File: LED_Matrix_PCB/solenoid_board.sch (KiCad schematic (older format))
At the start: 93 parts, among them J2 MCU_LEFT_LEGS, J3 MCU_RIGHT_LEGS

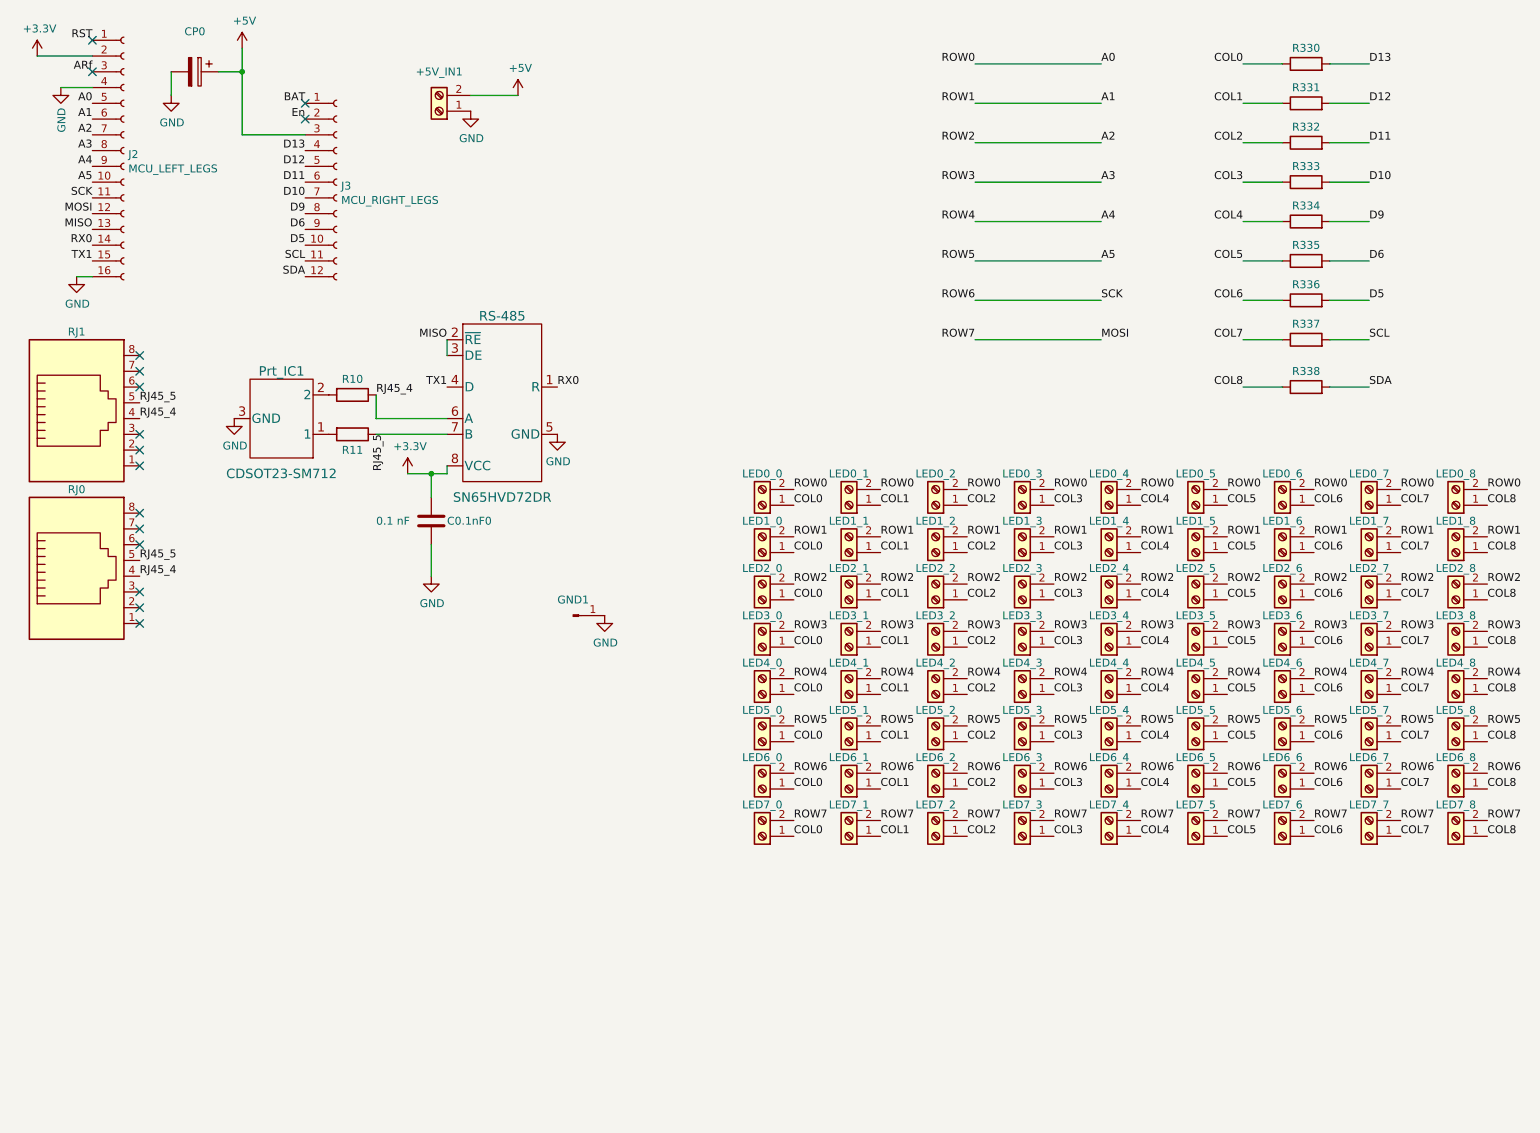
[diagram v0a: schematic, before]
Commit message: Forgot to close files before pushing.
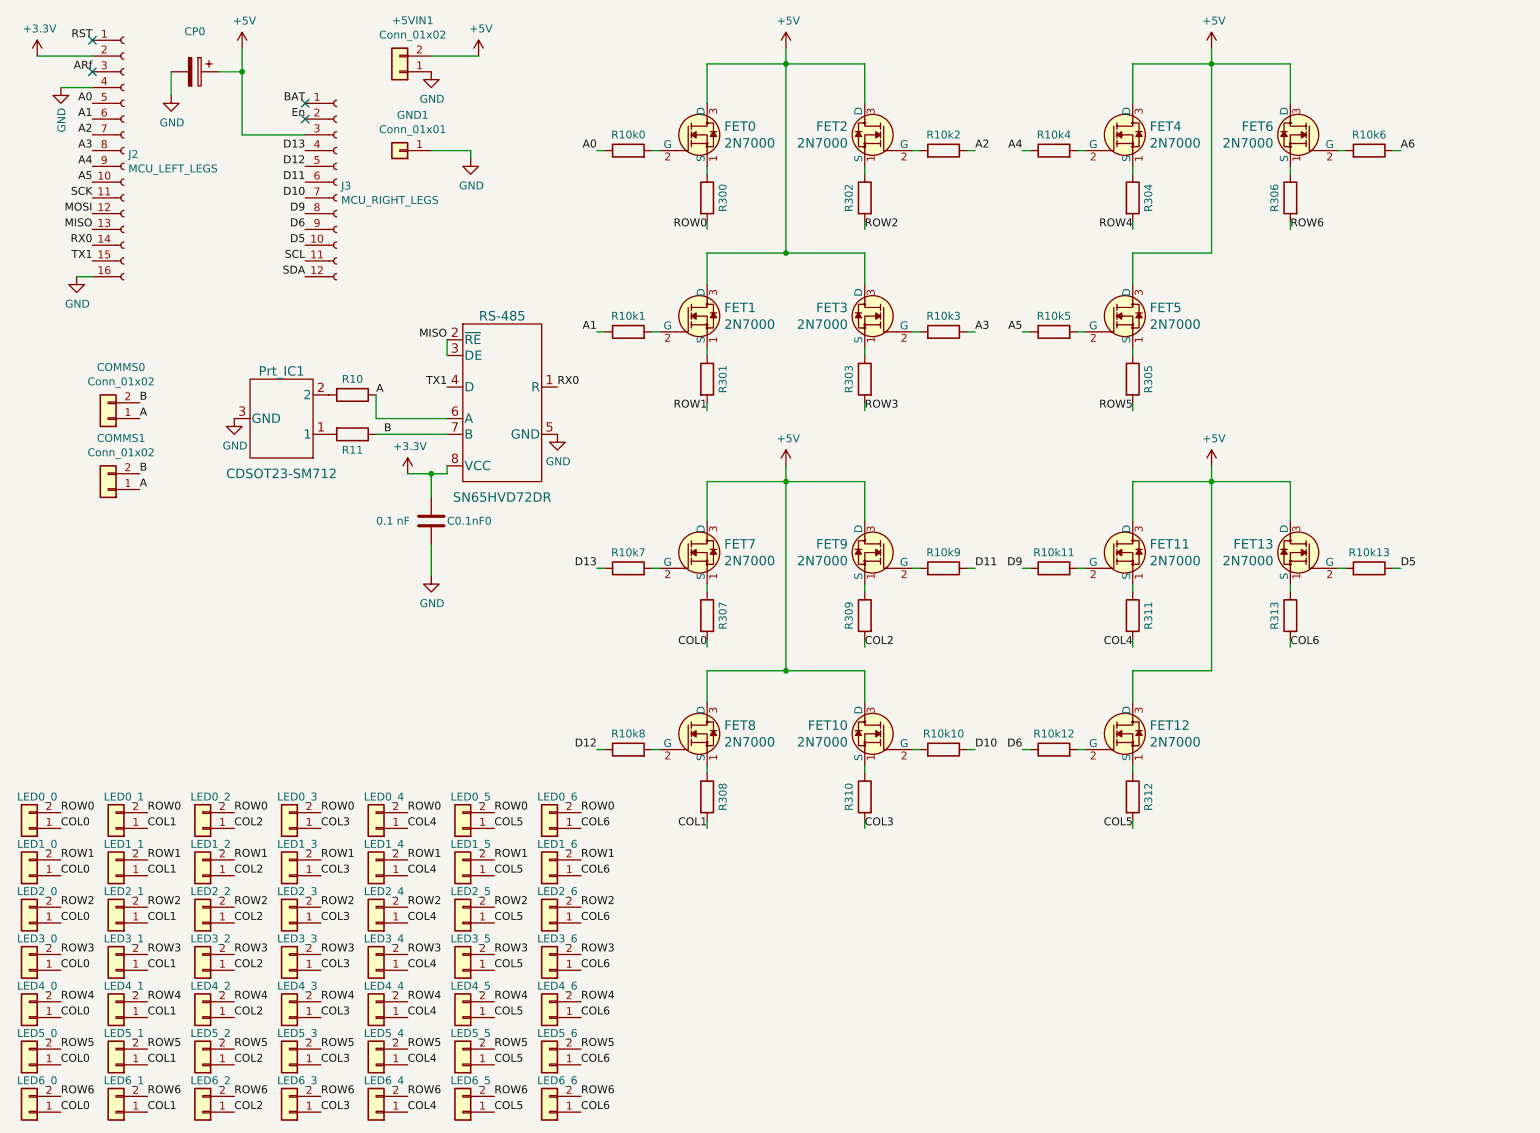
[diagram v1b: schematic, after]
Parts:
- removed +5V_IN1: MCU_PWR_Supply, TerminalBlock:TerminalBlock_bornier-2_P5.08mm, symbol Connector:Screw_Terminal_01x02
- removed GND1: Conn_01x01_Male, Connector_PinHeader_2.54mm:PinHeader_1x01_P2.54mm_Vertical, symbol Connector:Conn_01x01_Male
- removed LED0_0, LED0_1, LED0_2, LED0_3, LED0_4, LED0_5, LED0_6, LED0_7, LED0_8, LED1_0, LED1_1, LED1_2, LED1_3, LED1_4, LED1_5, LED1_6, LED1_7, LED1_8, LED2_0, LED2_1, LED2_2, LED2_3, LED2_4, LED2_5, LED2_6, LED2_7, LED2_8, LED3_0, LED3_1, LED3_2, LED3_3, LED3_4, LED3_5, LED3_6, LED3_7, LED3_8, LED4_0, LED4_1, LED4_2, LED4_3, LED4_4, LED4_5, LED4_6, LED4_7, LED4_8, LED5_0, LED5_1, LED5_2, LED5_3, LED5_4, LED5_5, LED5_6, LED5_7, LED5_8, LED6_0, LED6_1, LED6_2, LED6_3, LED6_4, LED6_5, LED6_6, LED6_7, LED6_8, LED7_0, LED7_1, LED7_2, LED7_3, LED7_4, LED7_5, LED7_6, LED7_7, LED7_8: Screw-terminal, TerminalBlock:TerminalBlock_bornier-2_P5.08mm, symbol Connector:Screw_Terminal_01x02
- removed R330, R331, R332: 330, Resistor_THT:R_Axial_DIN0309_L9.0mm_D3.2mm_P20.32mm_Horizontal, symbol Device:R
- removed R333, R334, R335, R336, R337, R338: R, Resistor_THT:R_Axial_DIN0309_L9.0mm_D3.2mm_P20.32mm_Horizontal, symbol Device:R
- removed RJ0, RJ1: RJ45, Connector_RJ:RJ45_Amphenol_54602-x08_Horizontal, symbol Connector:RJ45
- added +5VIN1, COMMS0, COMMS1, LED0_0, LED0_1, LED0_2, LED0_3, LED0_4, LED0_5, LED0_6, LED1_0, LED1_1, LED1_2, LED1_3, LED1_4, LED1_5, LED1_6, LED2_0, LED2_1, LED2_2, LED2_3, LED2_4, LED2_5, LED2_6, LED3_0, LED3_1, LED3_2, LED3_3, LED3_4, LED3_5, LED3_6, LED4_0, LED4_1, LED4_2, LED4_3, LED4_4, LED4_5, LED4_6, LED5_0, LED5_1, LED5_2, LED5_3, LED5_4, LED5_5, LED5_6, LED6_0, LED6_1, LED6_2, LED6_3, LED6_4, LED6_5, LED6_6: Conn_01x02, Connector_PinHeader_2.54mm:PinHeader_1x02_P2.54mm_Vertical, symbol Connector_Generic:Conn_01x02
- added FET0, FET1, FET10, FET11, FET12, FET13, FET2, FET3, FET4, FET5, FET6, FET7, FET8, FET9: 2N7000, digikey-footprints:TO-92-3, symbol dk_Transistors-FETs-MOSFETs-Single:2N7000
- added GND1: Conn_01x01, Connector_PinHeader_2.54mm:PinHeader_1x01_P2.54mm_Vertical, symbol Connector_Generic:Conn_01x01
- added R10k0, R10k1, R10k10, R10k11, R10k12, R10k13, R10k2, R10k3, R10k4, R10k5, R10k6, R10k7, R10k8, R10k9: 10k, Resistor_THT:R_Axial_DIN0204_L3.6mm_D1.6mm_P5.08mm_Vertical, symbol Device:R
- added R300, R301, R302, R303, R304, R305, R306, R307, R308, R309, R310, R311, R312, R313: 300, Resistor_THT:R_Axial_DIN0204_L3.6mm_D1.6mm_P5.08mm_Vertical, symbol Device:R
- R10, R11: footprint Resistor_THT:R_Axial_DIN0309_L9.0mm_D3.2mm_P20.32mm_Horizontal -> Resistor_THT:R_Axial_DIN0204_L3.6mm_D1.6mm_P7.62mm_Horizontal
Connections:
- net +5V: now also +5VIN1.2 (Pin_2), FET0.3 (D), FET1.3 (D), FET10.3 (D), FET11.3 (D), FET12.3 (D), FET13.3 (D), FET2.3 (D), FET3.3 (D), FET4.3 (D), FET5.3 (D), FET6.3 (D), FET7.3 (D), FET8.3 (D), FET9.3 (D)
- net A0: now also R10k0.1
- net A1: now also R10k1.1
- net A2: now also R10k2.1
- net A3: now also R10k3.1
- net A4: now also R10k4.1
- net A5: now also R10k5.1
- net COL0: now also LED0_0.1 (Pin_1), LED1_0.1 (Pin_1), LED2_0.1 (Pin_1), LED3_0.1 (Pin_1), LED4_0.1 (Pin_1), LED5_0.1 (Pin_1), LED6_0.1 (Pin_1), R307.2
- net COL1: now also LED0_1.1 (Pin_1), LED1_1.1 (Pin_1), LED2_1.1 (Pin_1), LED3_1.1 (Pin_1), LED4_1.1 (Pin_1), LED5_1.1 (Pin_1), LED6_1.1 (Pin_1), R308.2
- net COL2: now also LED0_2.1 (Pin_1), LED1_2.1 (Pin_1), LED2_2.1 (Pin_1), LED3_2.1 (Pin_1), LED4_2.1 (Pin_1), LED5_2.1 (Pin_1), LED6_2.1 (Pin_1), R309.2
- net COL3: now also LED0_3.1 (Pin_1), LED1_3.1 (Pin_1), LED2_3.1 (Pin_1), LED3_3.1 (Pin_1), LED4_3.1 (Pin_1), LED5_3.1 (Pin_1), LED6_3.1 (Pin_1), R310.2
- net COL4: now also LED0_4.1 (Pin_1), LED1_4.1 (Pin_1), LED2_4.1 (Pin_1), LED3_4.1 (Pin_1), LED4_4.1 (Pin_1), LED5_4.1 (Pin_1), LED6_4.1 (Pin_1), R311.2
- net COL5: now also LED0_5.1 (Pin_1), LED1_5.1 (Pin_1), LED2_5.1 (Pin_1), LED3_5.1 (Pin_1), LED4_5.1 (Pin_1), LED5_5.1 (Pin_1), LED6_5.1 (Pin_1), R312.2
- net COL6: now also LED0_6.1 (Pin_1), LED1_6.1 (Pin_1), LED2_6.1 (Pin_1), LED3_6.1 (Pin_1), LED4_6.1 (Pin_1), LED5_6.1 (Pin_1), LED6_6.1 (Pin_1), R313.2
- net D10: now also R10k10.1
- net D11: now also R10k9.1
- net D12: now also R10k8.1
- net D13: now also R10k7.1
- net D5: now also R10k13.1
- net D6: now also R10k12.1
- net D9: now also R10k11.1
- net GND: now also +5VIN1.1 (Pin_1), GND1.1 (Pin_1)
- net ROW6: now also LED6_0.2 (Pin_2), LED6_1.2 (Pin_2), LED6_2.2 (Pin_2), LED6_3.2 (Pin_2), LED6_4.2 (Pin_2), LED6_5.2 (Pin_2), LED6_6.2 (Pin_2), R306.2; no longer J2.11 (Pin_11)
- net RJ45_4 renamed A
- net A: now also COMMS0.1 (Pin_1), COMMS1.1 (Pin_1)
- net RJ45_5 renamed B
- net B: now also COMMS0.2 (Pin_2), COMMS1.2 (Pin_2)
- new net: FET0.1 (S), R300.1
- new net: FET0.2 (G), R10k0.2
- new net: FET1.1 (S), R301.1
- new net: FET1.2 (G), R10k1.2
- new net: FET2.1 (S), R302.1
- new net: FET2.2 (G), R10k2.2
- new net: FET3.1 (S), R303.1
- new net: FET3.2 (G), R10k3.2
- new net: FET4.1 (S), R304.1
- new net: FET4.2 (G), R10k4.2
- new net: FET5.1 (S), R305.1
- new net: FET5.2 (G), R10k5.2
- new net: FET6.1 (S), R306.1
- new net: FET6.2 (G), R10k6.2
- new net: FET7.1 (S), R307.1
- new net: FET7.2 (G), R10k7.2
- new net: FET8.1 (S), R308.1
- new net: FET8.2 (G), R10k8.2
- new net: FET9.1 (S), R309.1
- new net: FET9.2 (G), R10k9.2
- new net: FET10.1 (S), R310.1
- new net: FET10.2 (G), R10k10.2
- new net: FET11.1 (S), R311.1
- new net: FET11.2 (G), R10k11.2
- new net: FET12.1 (S), R312.1
- new net: FET12.2 (G), R10k12.2
- new net: FET13.1 (S), R313.1
- new net: FET13.2 (G), R10k13.2
- new net A6: R10k6.1
- new net ROW0: LED0_0.2 (Pin_2), LED0_1.2 (Pin_2), LED0_2.2 (Pin_2), LED0_3.2 (Pin_2), LED0_4.2 (Pin_2), LED0_5.2 (Pin_2), LED0_6.2 (Pin_2), R300.2
- new net ROW1: LED1_0.2 (Pin_2), LED1_1.2 (Pin_2), LED1_2.2 (Pin_2), LED1_3.2 (Pin_2), LED1_4.2 (Pin_2), LED1_5.2 (Pin_2), LED1_6.2 (Pin_2), R301.2
- new net ROW2: LED2_0.2 (Pin_2), LED2_1.2 (Pin_2), LED2_2.2 (Pin_2), LED2_3.2 (Pin_2), LED2_4.2 (Pin_2), LED2_5.2 (Pin_2), LED2_6.2 (Pin_2), R302.2
- new net ROW3: LED3_0.2 (Pin_2), LED3_1.2 (Pin_2), LED3_2.2 (Pin_2), LED3_3.2 (Pin_2), LED3_4.2 (Pin_2), LED3_5.2 (Pin_2), LED3_6.2 (Pin_2), R303.2
- new net ROW4: LED4_0.2 (Pin_2), LED4_1.2 (Pin_2), LED4_2.2 (Pin_2), LED4_3.2 (Pin_2), LED4_4.2 (Pin_2), LED4_5.2 (Pin_2), LED4_6.2 (Pin_2), R304.2
- new net ROW5: LED5_0.2 (Pin_2), LED5_1.2 (Pin_2), LED5_2.2 (Pin_2), LED5_3.2 (Pin_2), LED5_4.2 (Pin_2), LED5_5.2 (Pin_2), LED5_6.2 (Pin_2), R305.2
- new net SCK: J2.11 (Pin_11)
- no-connect marks 16 -> 4
